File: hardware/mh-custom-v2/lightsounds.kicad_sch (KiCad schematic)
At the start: 26 parts, among them J1 Conn_01x03_Male, J2 Conn_01x03_Female, SW1 SW_DIP_x04, T1 AO3400A, T2 AO3400A, T5 AO3400A, T6 AO3400A

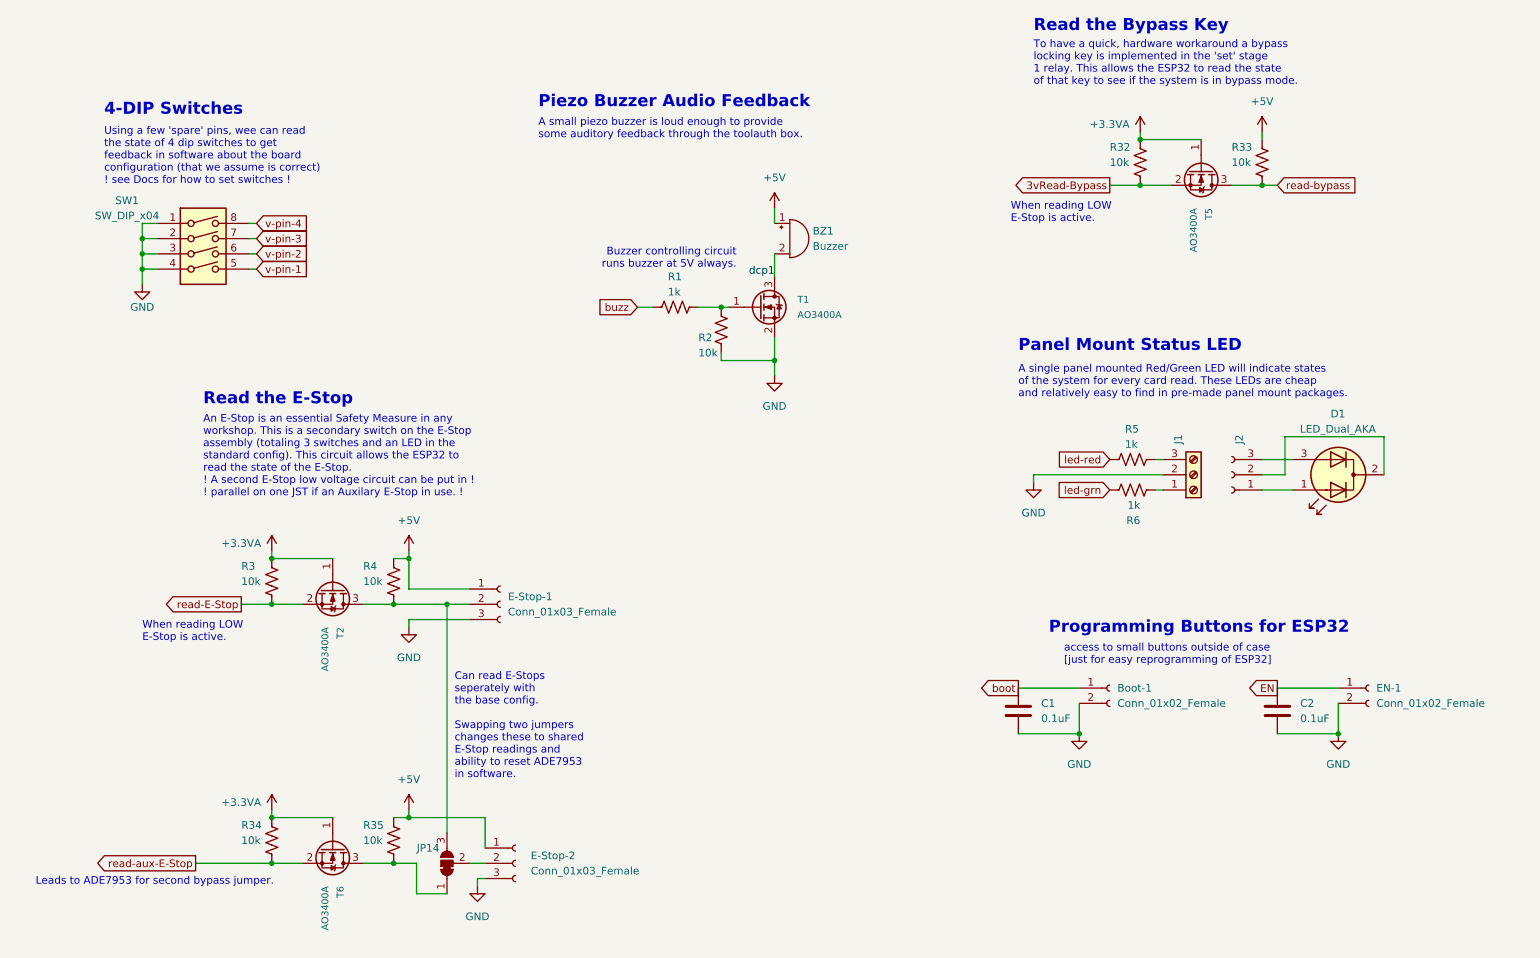
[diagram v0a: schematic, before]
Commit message: just ordered from JLCPCB
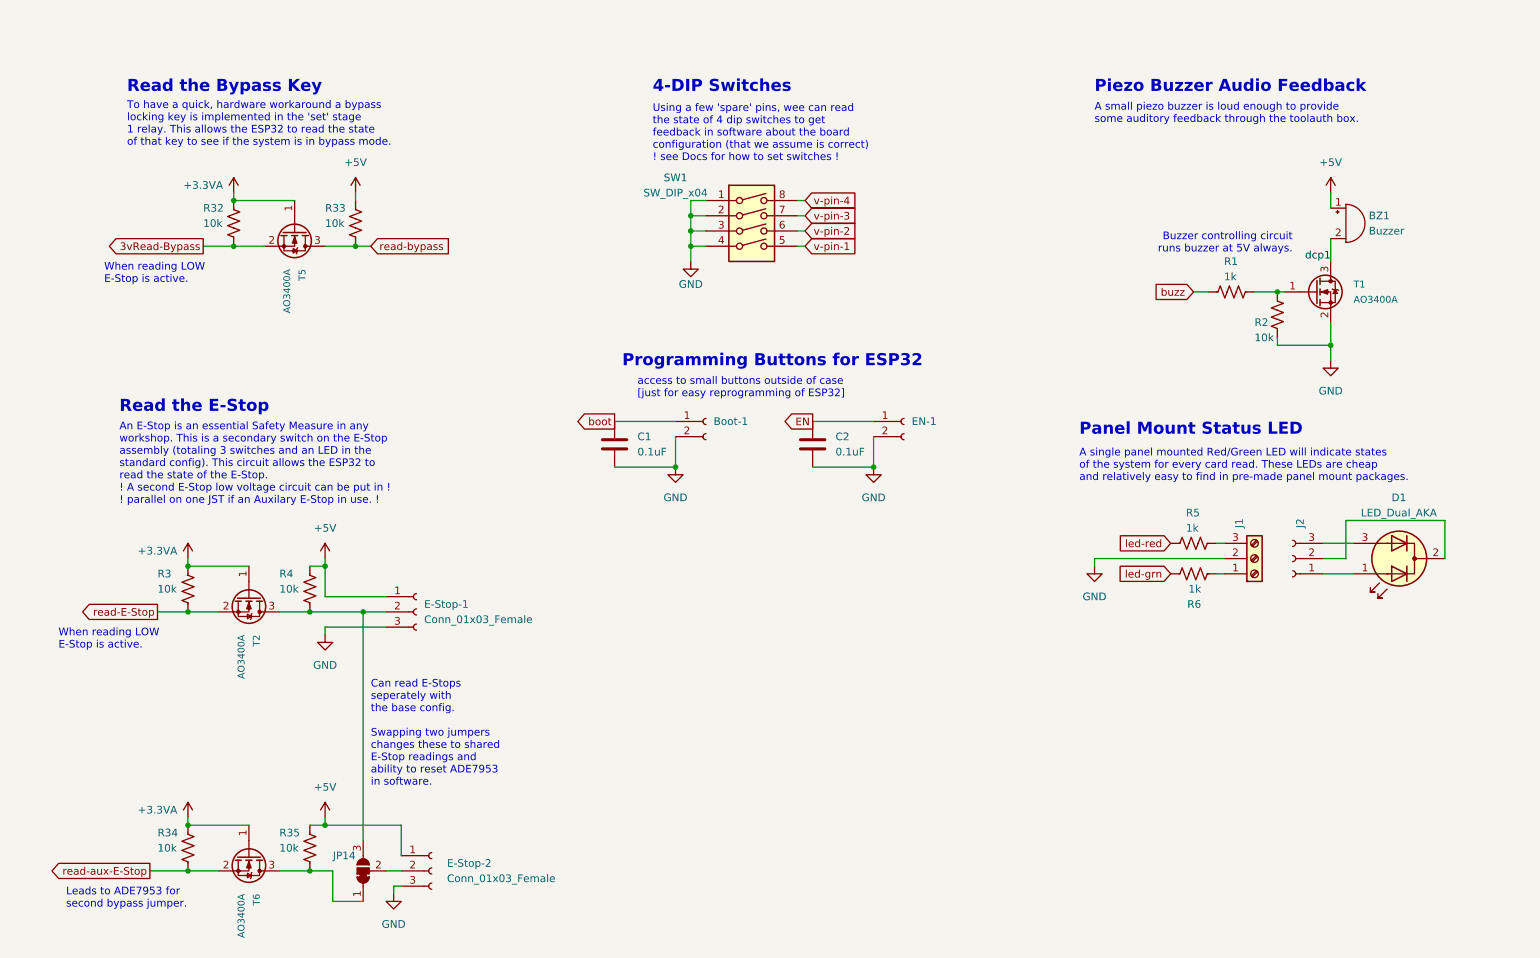
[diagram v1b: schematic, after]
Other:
- company: (none) -> Corey Rice & MakeHaven
- title: (none) -> Onboard Lights, Sounds and Logic Level Converters
- moved on the sheet: BZ1, Boot-1, C1, C2, D1, E-Stop-1, E-Stop-2, EN-1, J1, J2, JP14, R1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
